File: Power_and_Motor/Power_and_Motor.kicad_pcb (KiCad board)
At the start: 2 copper layers, 110 x 110 mm, 25 parts, among them J1 Barrel_Jack_Switch_Pin3Ring, M1 Motor_DC, Q1 BC337, Q2 BC337, SW1 SW_DPDT_x2, U1 LM317_TO-220, U2 Pin-Connector, U3 Pin-Connector, U4 Pin-Connector, U5 Pin-Connector, U6 Pin-Connector, U7 Pin-Connector

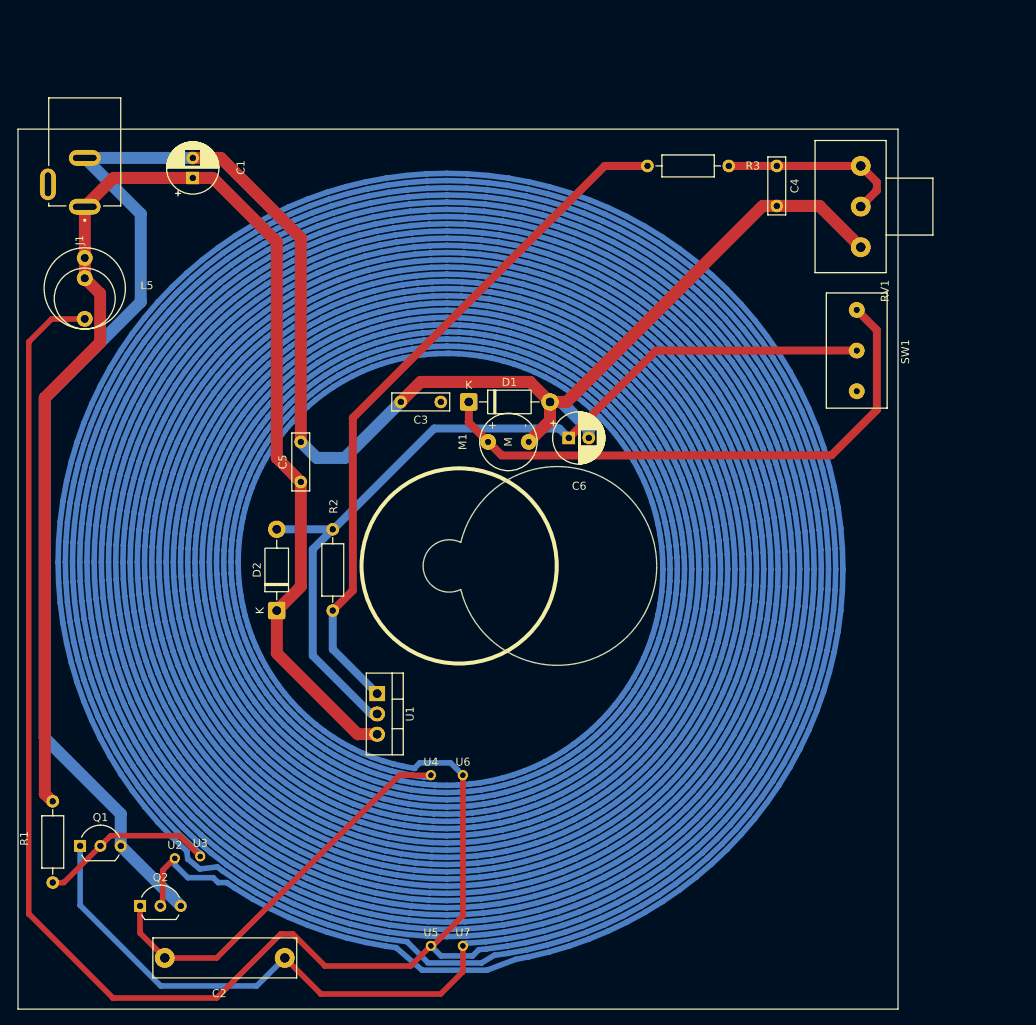
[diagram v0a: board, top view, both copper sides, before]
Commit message: ReworkPM2
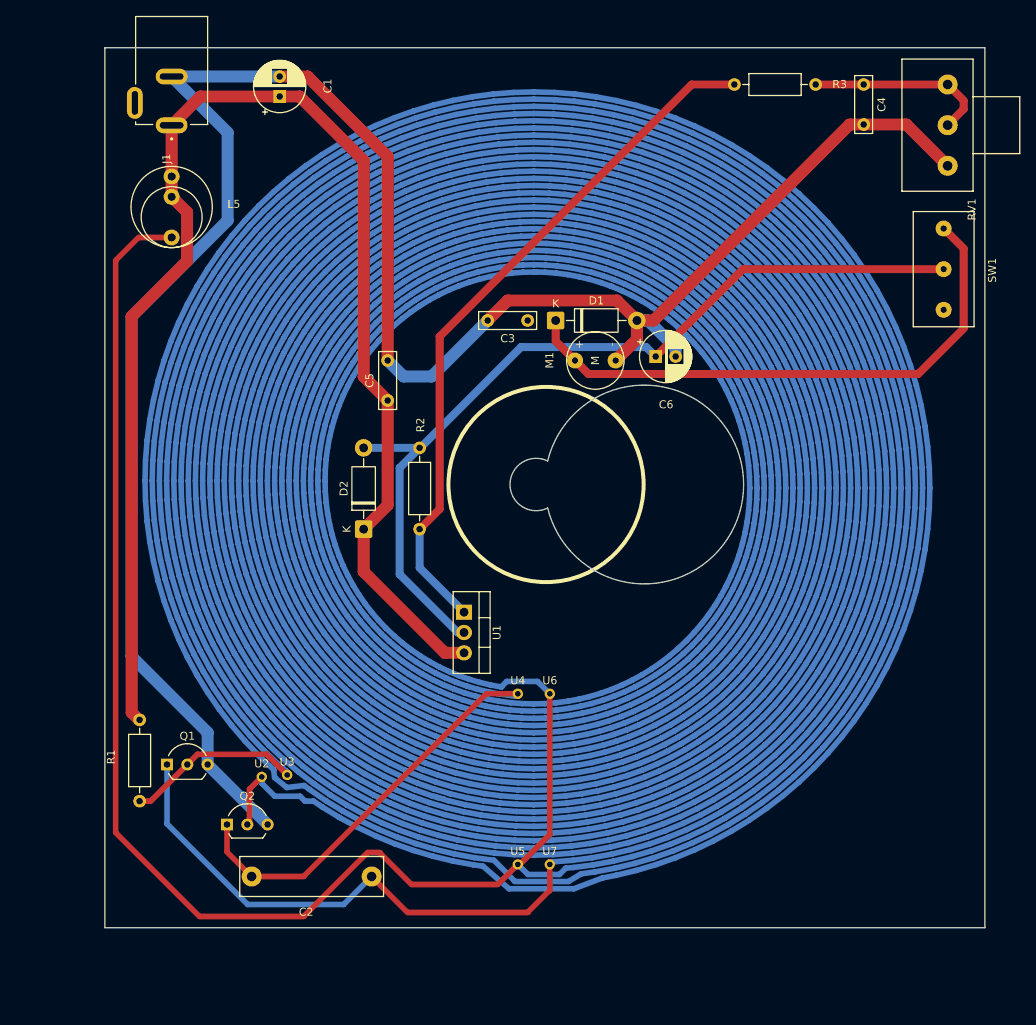
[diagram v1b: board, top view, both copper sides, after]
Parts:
- moved C2 14.9 mm to (121.9, 149.3)
- moved L5 14.9 mm to (104.4, 65.6)
- moved Q1 14.9 mm to (103.8, 135.3)
- moved Q2 14.9 mm to (111.3, 142.8)
- moved R2 14.9 mm to (135.4, 95.7)
- moved U3 14.9 mm to (118.8, 136.6)
- moved U5 14.9 mm to (147.6, 147.8)
- moved U7 14.9 mm to (151.6, 147.8)
- moved C1 14.9 mm to (117.9, 51.8)
- moved C4 14.9 mm to (190.9, 50.3)
- moved J1 14.9 mm to (104.4, 49.3)
- moved R3 14.9 mm to (174.7, 50.3)
- moved RV1 14.9 mm to (201.4, 55.4)
- moved C3 14.9 mm to (148.9, 79.8)
- moved C5 14.9 mm to (131.4, 89.8)
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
